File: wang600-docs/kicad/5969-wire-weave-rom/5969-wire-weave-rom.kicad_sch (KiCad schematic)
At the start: 39 parts, among them Q32 GT644, Q33 GT644, Q34 2N3640, U11 7426, U36 SP380A, U38 74LS04

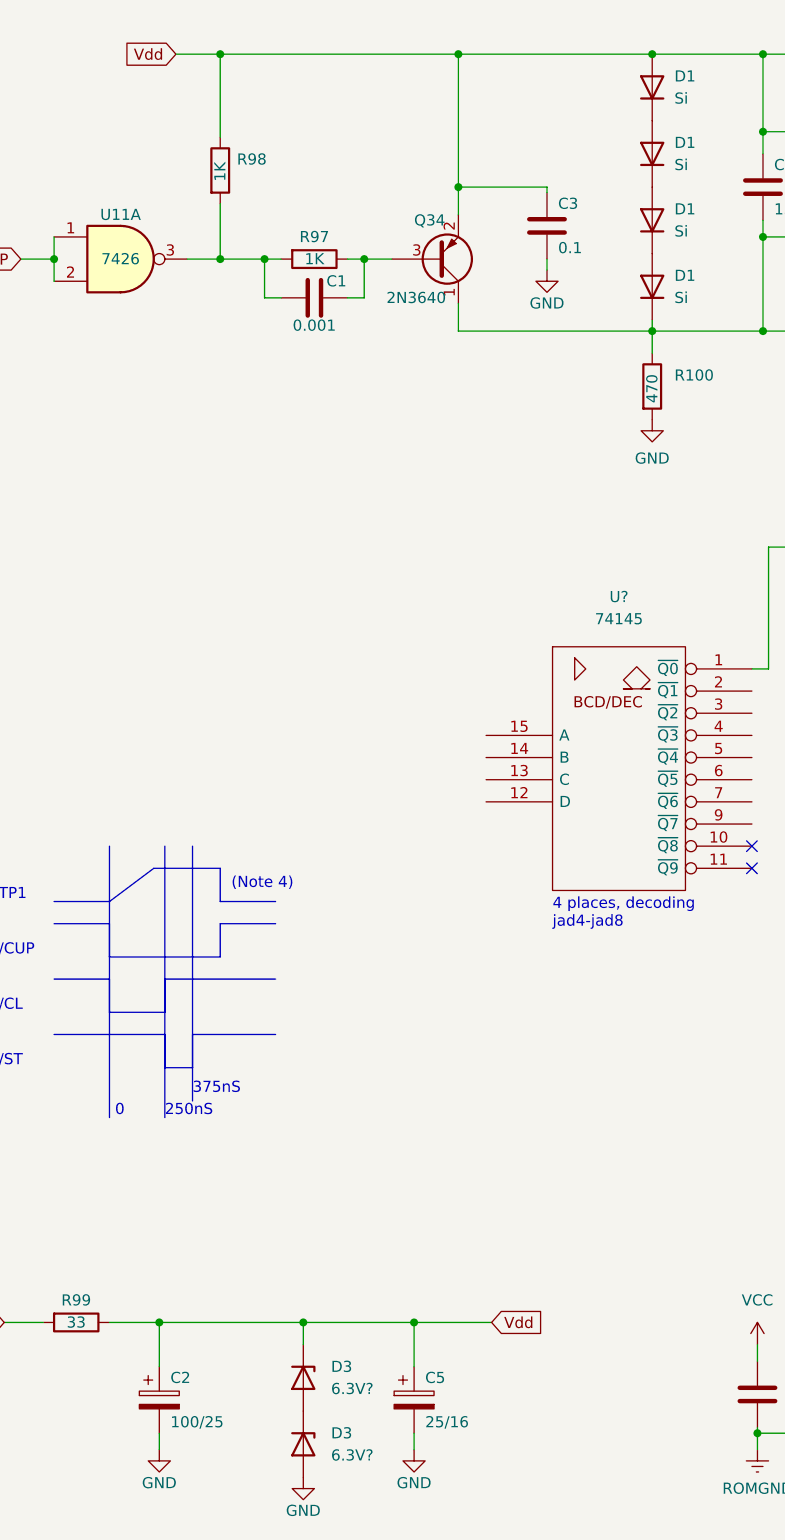
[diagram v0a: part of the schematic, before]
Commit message: cleanup schematics
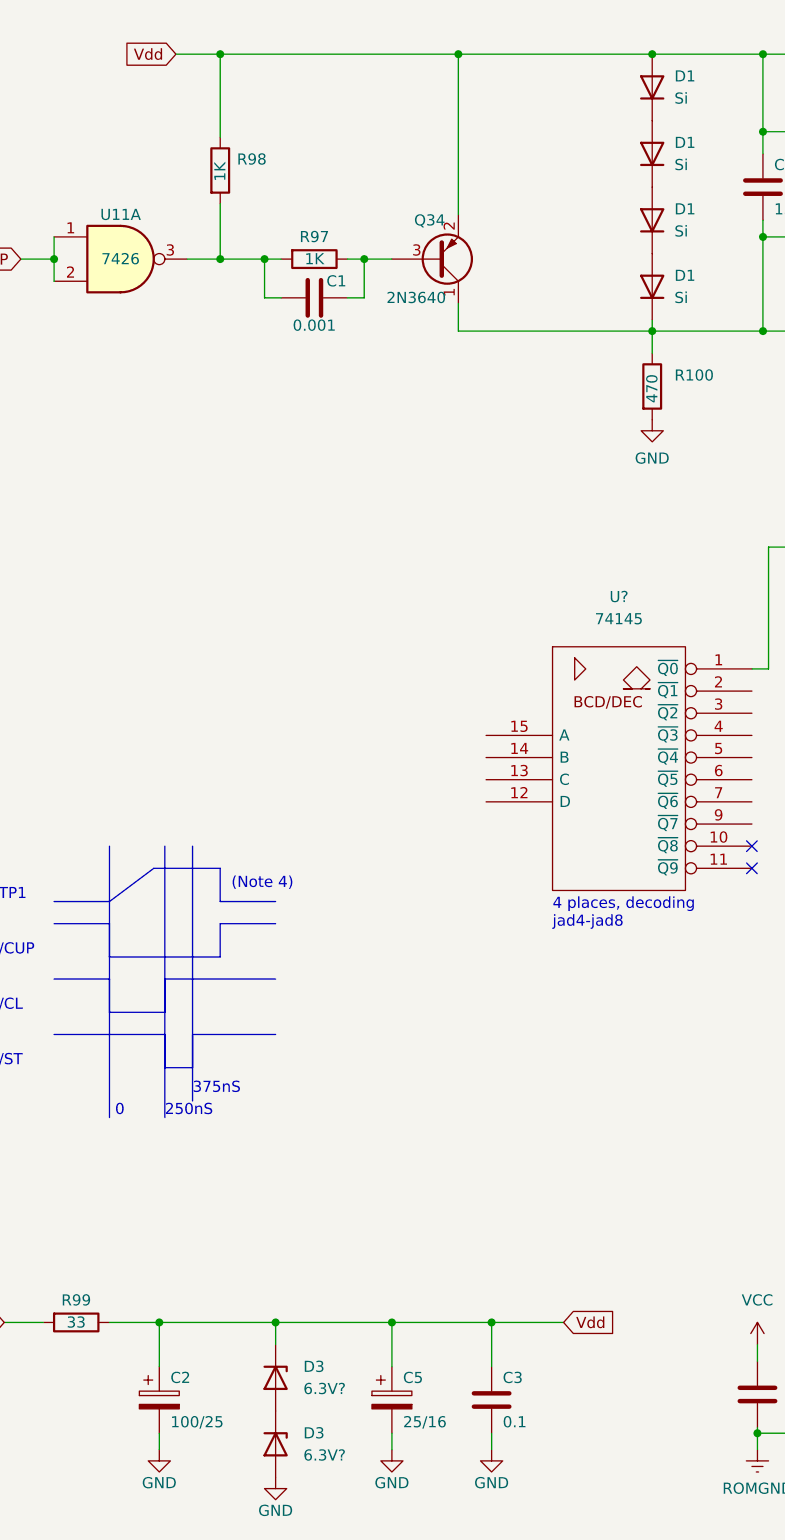
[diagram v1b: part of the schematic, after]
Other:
- moved on the sheet: C3, C5, D3
